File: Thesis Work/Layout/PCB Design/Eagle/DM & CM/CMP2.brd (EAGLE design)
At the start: 48.1 x 19.5 mm, 7 parts, among them J1 SMA-J-P-H-ST-EM1, J2 SMA-J-P-H-ST-EM1

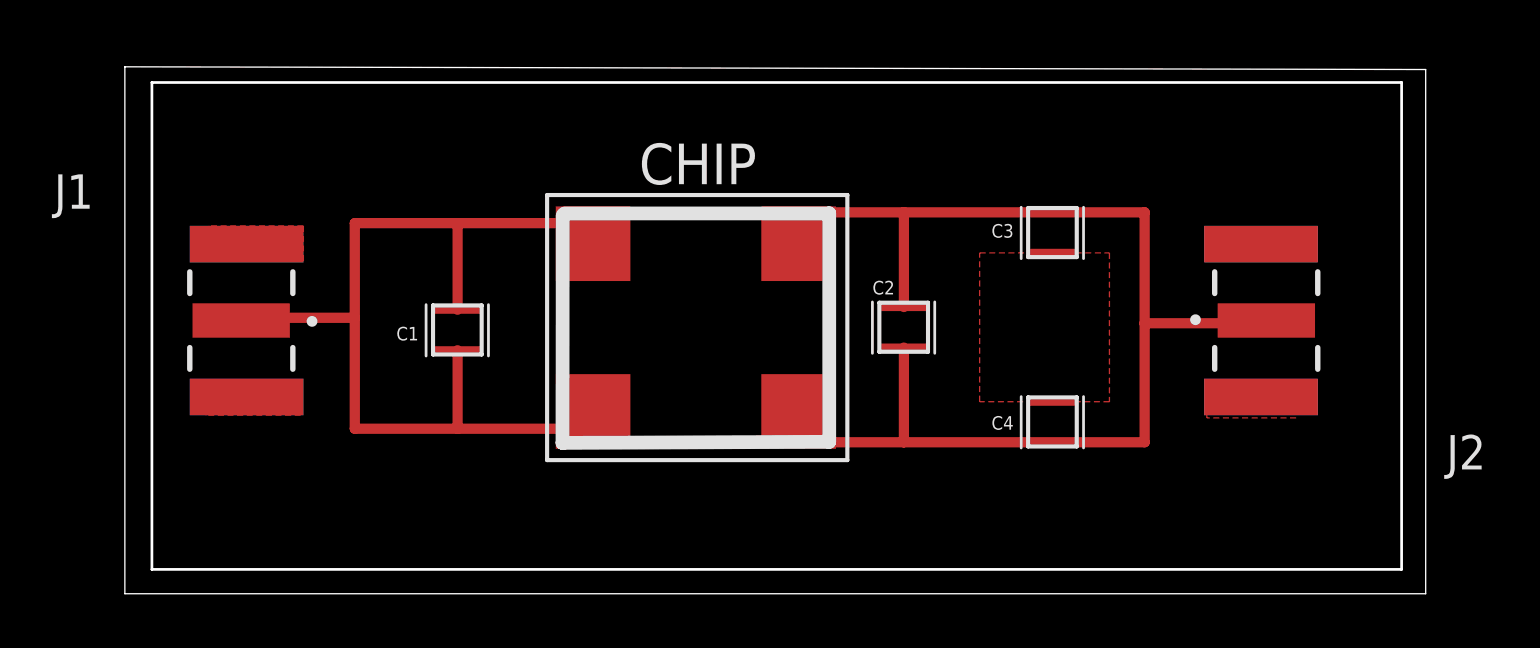
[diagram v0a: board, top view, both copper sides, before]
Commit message: c
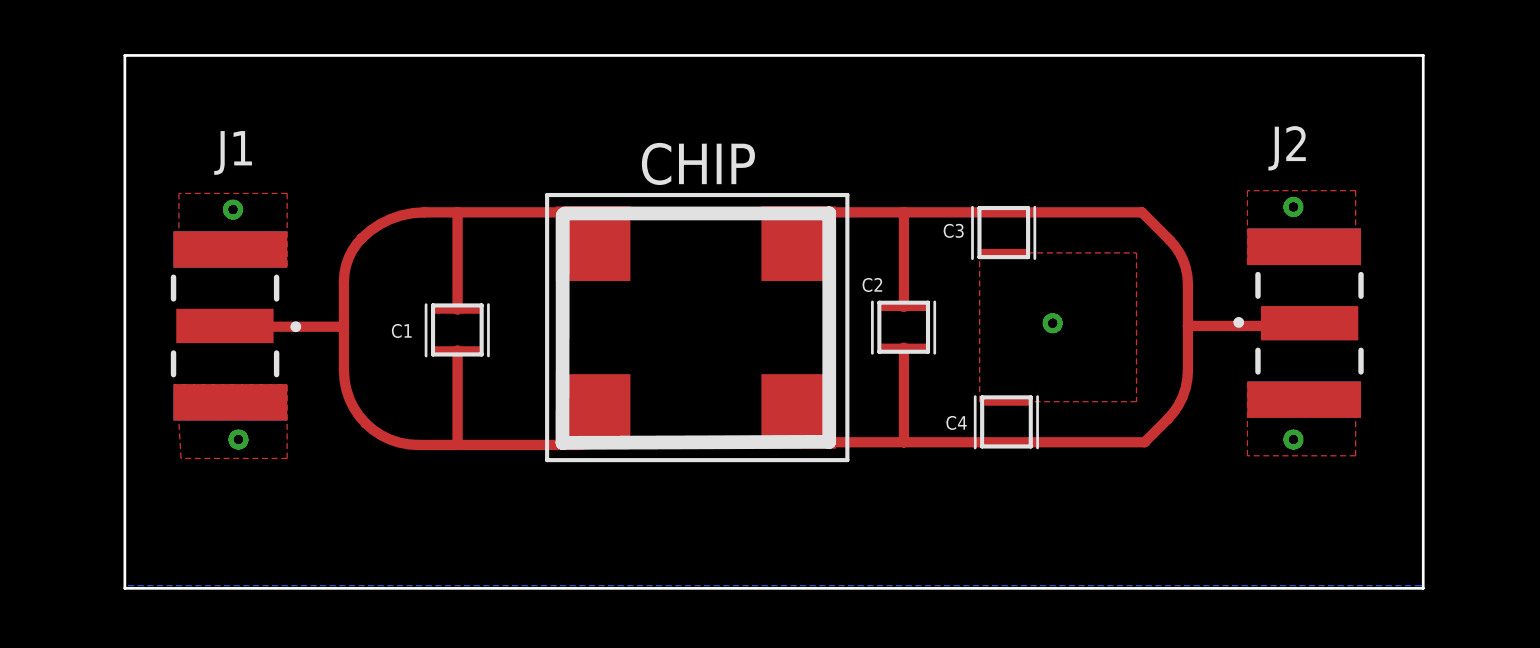
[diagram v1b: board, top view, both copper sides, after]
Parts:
- moved C3 1.80 mm to (50.2, 26.1)
- moved C4 1.70 mm to (50.3, 19.1)
- moved J2 1.60 mm to (61.5, 22.7)
- moved J1 0.63 mm to (21.4, 22.6)
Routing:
- net N$4: track 45.7 -> 46.6 mm
- added copper zone on layer 16, net GND
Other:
- board size 48.1 x 19.5 mm -> 48 x 19.7 mm
